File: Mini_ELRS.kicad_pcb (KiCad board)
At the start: 4 copper layers, 26.7 x 15.8 mm, 30 parts, among them J1 Conn_01x02, J2 Conn_01x03_MountingPin, J3 Conn_01x04, J4 Conn_01x03_MountingPin, J5 Conn_01x03_MountingPin, J6 Conn_01x03_MountingPin, Q1 Q_NMOS_GSD, Q2 Q_NMOS_GSD, U1 ESP32-PICO-D4, U2 TC2014-3.3VxCTTR, U3 SX1280IMLTRT, Y1 Crystal_GND24_Small

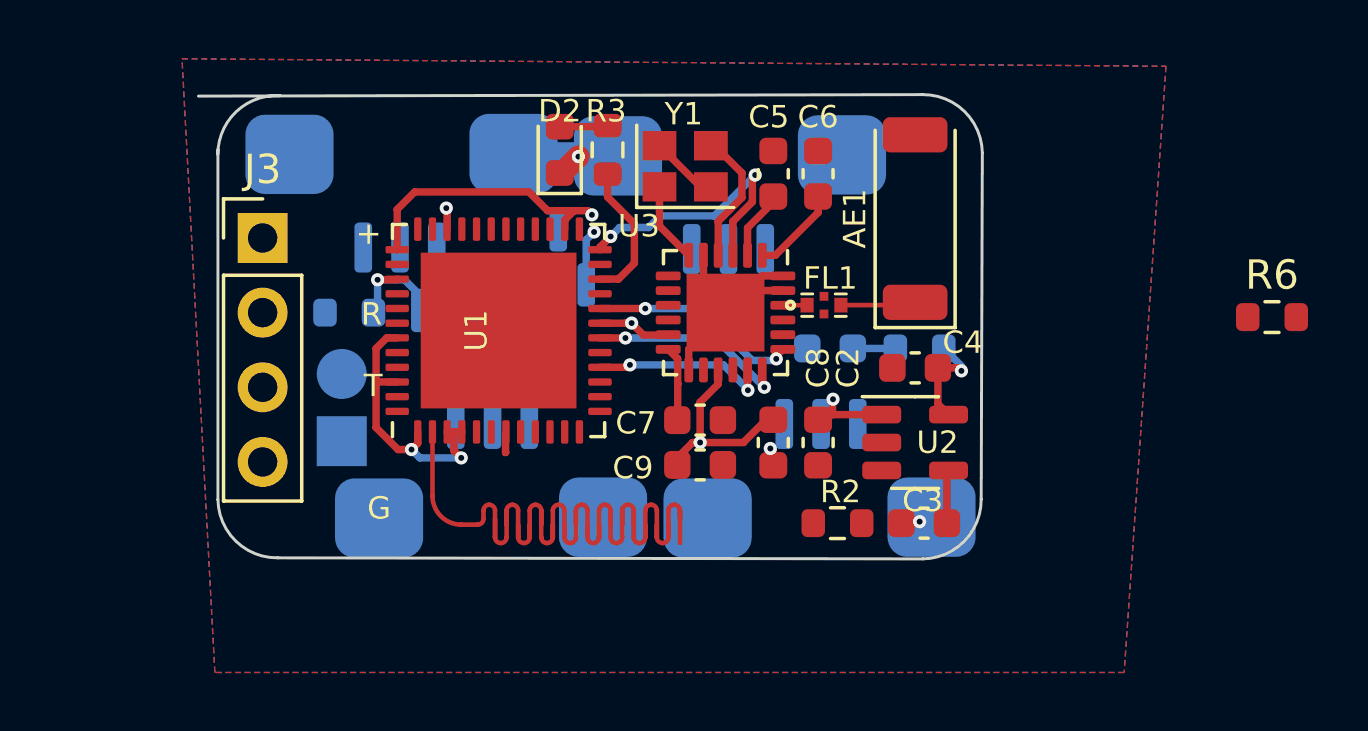
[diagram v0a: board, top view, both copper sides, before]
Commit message: finished TX mobile
Signed-off-by: huangzzk <huangcmzzk@gmail.com>
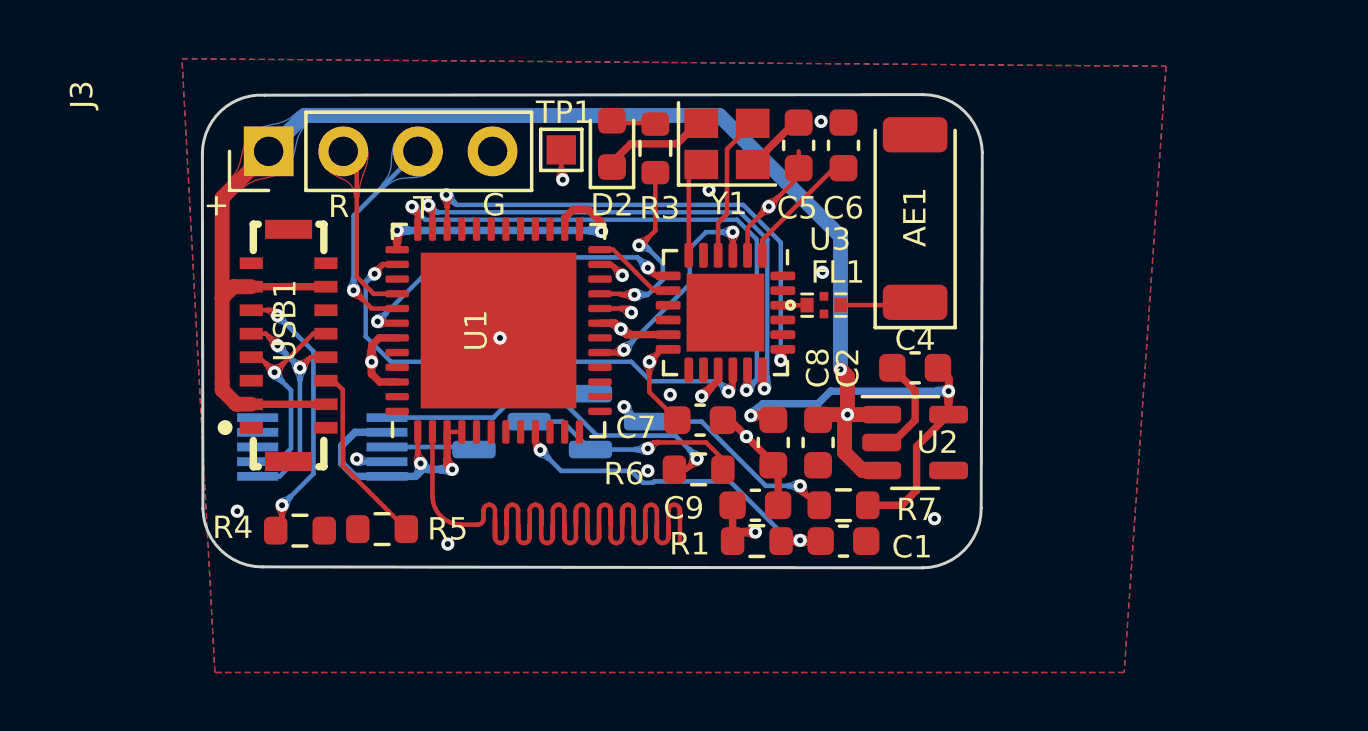
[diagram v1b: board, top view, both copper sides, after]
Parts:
- removed C3: 180pF, Capacitor_SMD:C_0603_1608Metric
- removed J1: Conn_01x02, Connector_PinHeader_2.54mm:PinHeader_2x01_P2.54mm_Vertical
- removed J2, J4, J5, J6: Conn_01x03_MountingPin, Connector_Molex:Molex_CLIK-Mate_502386-0370_1x03-1MP_P1.25mm_Horizontal
- removed R2: NC, Resistor_SMD:R_0603_1608Metric
- added R7: 10K, Resistor_SMD:R_0603_1608Metric, F.Cu at (119.7, 69.7)
- added TP1: TestPoint, TestPoint:TestPoint_Pad_1.0x1.0mm, F.Cu at (110.1, 57.6)
- added U4: CH340E, Package_SO:MSOP-10_3x3mm_P0.5mm, B.Cu at (102.0, 67.7)
- added USB1: 918-118A2021Y40002, ic_footprint:TYPE-C-SMD_JINGTUOJIN_918-118A2021Y40002, F.Cu at (100.9, 64.3)
- C1, R1, R4, R5: moved to F.Cu
- moved R6 20.2 mm to (114.8, 68.5), turned to 180 degrees
- moved R1 8.58 mm to (116.8, 70.9), turned to 0 degrees
- moved R5 7.88 mm to (104.0, 70.5)
- moved R4 7.60 mm to (101.2, 70.6)
- moved C1 6.57 mm to (119.7, 70.9), turned to 0 degrees
- moved Q2 5.95 mm to (112.1, 66.9), turned to 0 degrees
- moved Q1 3.38 mm to (108.1, 66.9), turned to 0 degrees
- moved J3 2.95 mm to (100.2, 57.7), turned to 90 degrees
- moved C9 2.33 mm to (116.7, 69.7)
- moved D2 1.79 mm to (111.9, 57.4)
- moved R3 1.63 mm to (113.3, 57.6)
- moved Y1 1.61 mm to (115.8, 57.4)
- moved C5 1.30 mm to (118.2, 57.5)
- moved C6 1.30 mm to (119.7, 57.5)
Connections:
- net +BATT renamed +5V
- Q1 pad 1: /PWM5 -> /CRSF_TX
- Q2 pad 1: /PWM3 -> Net-(Q1-Pad3)
- Q2 pad 3: Net-(J2-Pad3) -> /CRSF
- R4 pad 1: /PWM5 -> GND
- R4 pad 2: GND -> Net-(R4-Pad2)
- R5 pad 1: /PWM3 -> Net-(R5-Pad1)
- R6 pad 1: /NSS -> Net-(Q1-Pad3)
- R6 pad 2: GND -> /TNOW
- U1 pad 12: /PWM7 -> unconnected-(U1-Pad12)
- U1 pad 13: /PWM4 -> unconnected-(U1-Pad13)
- U1 pad 14: /PWM2 -> unconnected-(U1-Pad14)
- U1 pad 16: /MOSI -> unconnected-(U1-Pad16)
- U1 pad 17: unconnected-(U1-Pad17) -> /NRST
- U1 pad 18: /SCK -> unconnected-(U1-Pad18)
- U1 pad 20: /NSS -> /CRSF
- U1 pad 21: unconnected-(U1-Pad21) -> /LED
- U1 pad 22: /LED -> unconnected-(U1-Pad22)
- U1 pad 24: /NRST -> /DIO1
- U1 pad 28: /PWM1 -> unconnected-(U1-Pad28)
- U1 pad 34: /PWM3 -> /NSS
- U1 pad 35: unconnected-(U1-Pad35) -> /SCK
- U1 pad 36: /PWM6 -> /MOSI
- U1 pad 38: unconnected-(U1-Pad38) -> /MISO
- U1 pad 39: /PWM5 -> unconnected-(U1-Pad39)
- U1 pad 42: /PWM8 -> /BUSY
- U1 pad 5: /BUSY -> unconnected-(U1-Pad5)
- U1 pad 7: /DIO1 -> unconnected-(U1-Pad7)
- U1 pad 8: /MISO -> unconnected-(U1-Pad8)
- U2 pad 4: Net-(C3-Pad1) -> unconnected-(U2-Pad4)
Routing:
- net +5V: track 2.52 -> 49.1 mm, vias 1 -> 2
- net +3V3: track 42.9 -> 72.1 mm, vias 6 -> 11
- net /CRSF: track 0.00 -> 24.4 mm, vias 0 -> 4
- net /MISO: track 0.00 -> 17.1 mm, vias 0 -> 2
- net /MOSI: track 6.14 -> 19.0 mm
- net /TNOW: track 0.00 -> 12.5 mm, vias 0 -> 1
- net /SCK: track 6.91 -> 18.7 mm
- net /BUSY: track 0.00 -> 11.7 mm, vias 0 -> 2
- net Net-(C5-Pad1): track 4.70 -> 15.8 mm, vias 0 -> 2
- net Net-(C1-Pad1): track 1.45 -> 12.2 mm, vias 0 -> 2
- net /NSS: track 7.17 -> 17.6 mm
- net Net-(R4-Pad2): track 0.00 -> 9.32 mm, vias 0 -> 2
- net /PWM3: track 8.01 -> 0.00 mm, vias 2 -> 0
- net /DP: track 0.00 -> 7.89 mm, vias 0 -> 2
- net Net-(Q1-Pad3): track 0.00 -> 7.64 mm, vias 0 -> 1
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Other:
- board size 26.7 x 15.8 mm -> 26.5 x 16.1 mm
- board text removed: "PWM1"
- board text removed: "PWM2"
- board text removed: "PWM3"
- board text removed: "PWM4"
- board text removed: "PWM5"
